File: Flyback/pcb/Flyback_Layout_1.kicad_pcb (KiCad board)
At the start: 2 copper layers, 44 parts

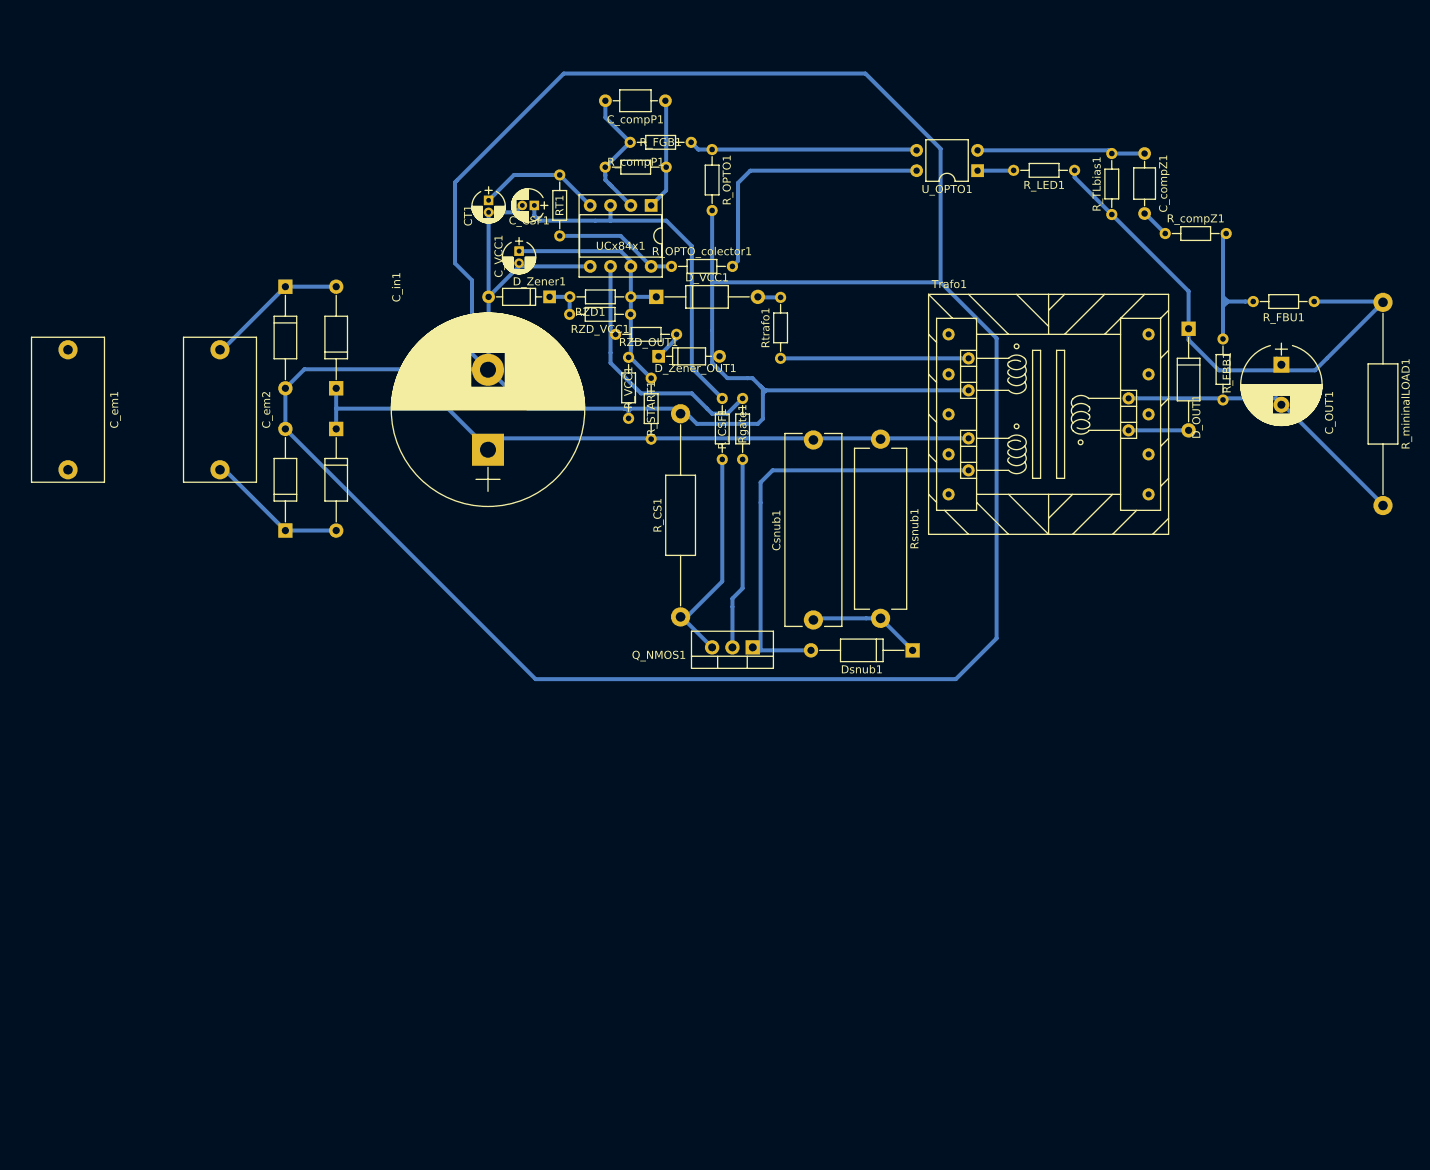
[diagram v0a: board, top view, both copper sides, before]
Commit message: add photo
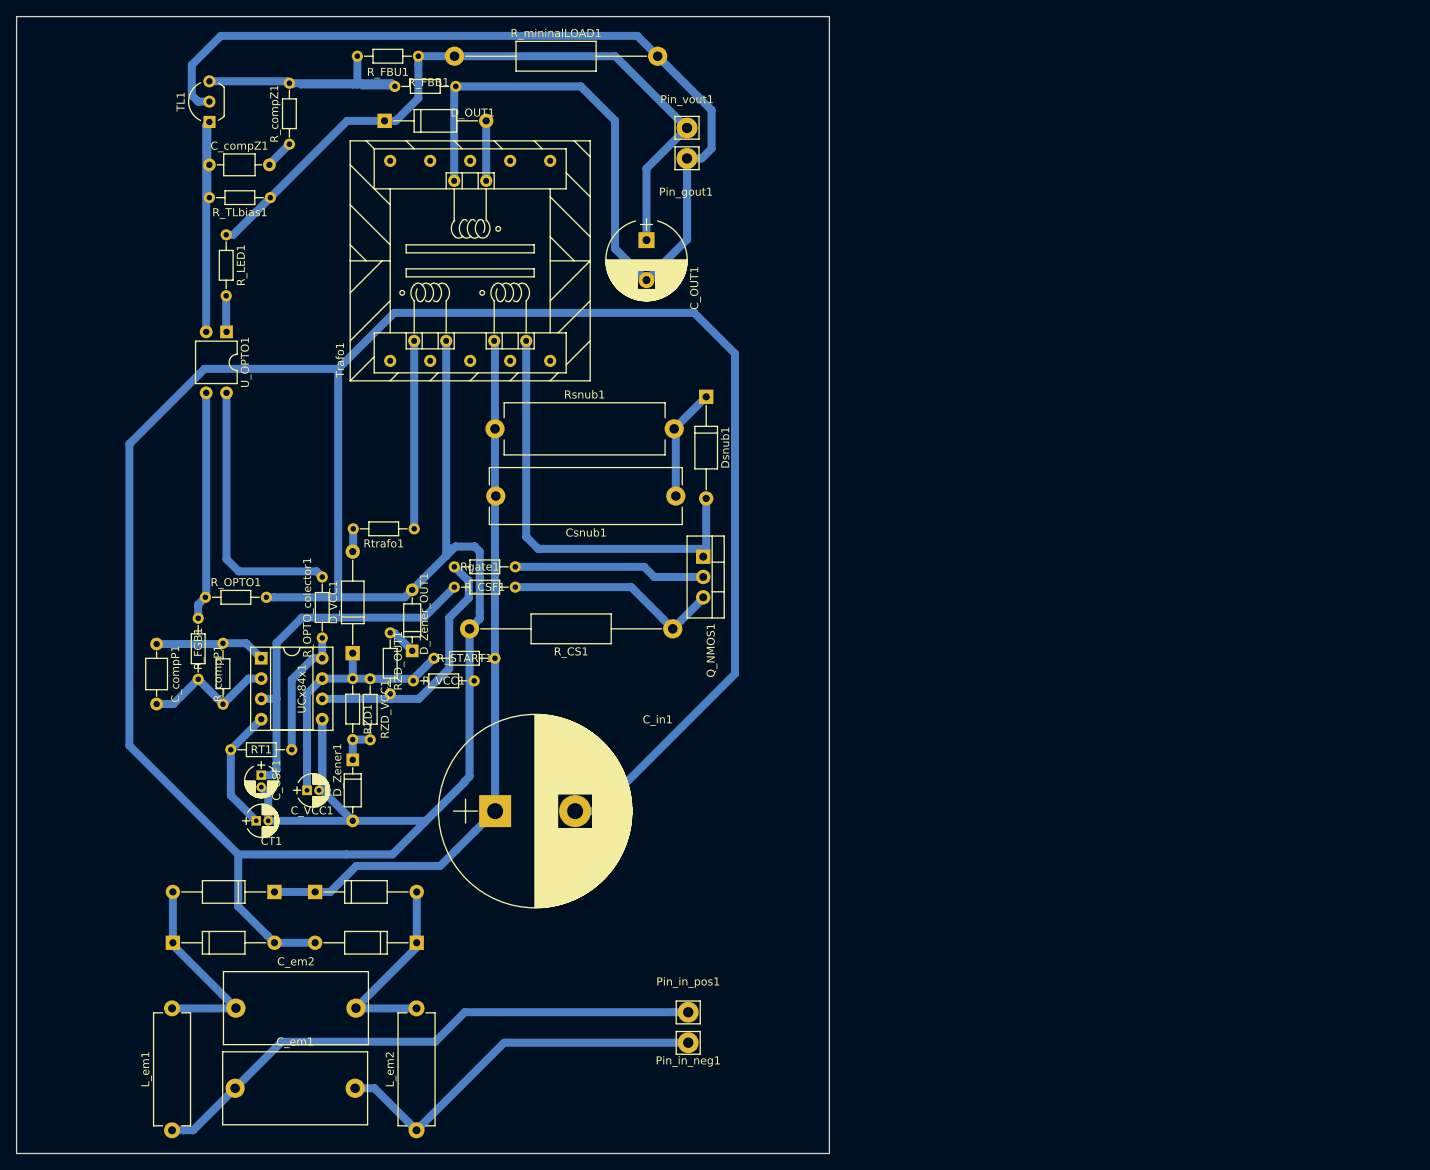
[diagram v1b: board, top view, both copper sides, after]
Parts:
- added L_em1: L, Inductors_THT:L_Axial_L14.0mm_D4.5mm_P15.24mm_Horizontal_Fastron_LACC, F.Cu at (75.4, 196.3)
- added L_em2: L, Inductors_THT:L_Axial_L14.0mm_D4.5mm_P15.24mm_Horizontal_Fastron_LACC, F.Cu at (105.9, 196.3)
- added Pin_gout1: CONN_01X01, Connectors:Pin_d1.4mm_L8.5mm_W2.8mm_FlatFork, F.Cu at (139.7, 74.8)
- added Pin_in_neg1: CONN_01X01, Connectors:Pin_d1.4mm_L8.5mm_W2.8mm_FlatFork, F.Cu at (139.9, 185.3)
- added Pin_in_pos1: CONN_01X01, Connectors:Pin_d1.4mm_L8.5mm_W2.8mm_FlatFork, F.Cu at (139.9, 181.5)
- added Pin_vout1: CONN_01X01, Connectors:Pin_d1.4mm_L8.5mm_W2.8mm_FlatFork, F.Cu at (139.7, 71.0)
- added TL1: Ajus_Shunt, TO_SOT_Packages_THT:TO-92_Inline_Wide, F.Cu at (80.0, 70.2)
- moved R_mininalLOAD1 120.1 mm to (110.7, 62.0), turned to 0 degrees
- moved C_compZ1 116.9 mm to (80.0, 75.6), turned to 0 degrees
- moved R_FBU1 116.1 mm to (98.5, 62.0)
- moved R_compZ1 110.0 mm to (90.0, 73.0), turned to 90 degrees
- moved R_LED1 106.4 mm to (82.1, 84.3), turned to 270 degrees
- moved R_TLbias1 105.2 mm to (87.7, 79.7), turned to 180 degrees
- moved D_OUT1 103.8 mm to (101.9, 70.1), turned to 0 degrees
- moved R_FBB1 103.6 mm to (110.8, 65.8), turned to 180 degrees
- moved U_OPTO1 96.0 mm to (82.2, 96.5), turned to 270 degrees
- moved C_em1 94.7 mm to (83.3, 191.0), turned to 0 degrees
- moved C_compP1 93.0 mm to (73.4, 135.5), turned to 270 degrees
- moved R_FGB1 86.1 mm to (78.6, 139.9), turned to 90 degrees
- moved R_OPTO1 84.5 mm to (79.5, 129.6), turned to 0 degrees
- moved Dret_1 83.2 mm to (75.5, 172.8), turned to 0 degrees
- moved CT1 82.8 mm to (85.9, 157.6), turned to 0 degrees
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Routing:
- net GOUT: track 37.3 -> 167.8 mm
- net Net-(C_em1-Pad1): track 0.00 -> 98.8 mm
- net VRET: track 88.7 -> 152.7 mm
- net Net-(C_em1-Pad2): track 0.00 -> 48.4 mm
- net GND: track 458.9 -> 499.2 mm
- net Net-(C_compZ1-Pad1): track 21.0 -> 52.8 mm
- net Net-(R_FBB1-Pad2): track 19.3 -> 46.7 mm
- net Net-(R_FGB1-Pad2): track 28.0 -> 53.6 mm
- net VOUT: track 65.2 -> 89.8 mm
- net ISENSE: track 45.1 -> 60.9 mm
- net VCC: track 33.3 -> 48.3 mm
- net Net-(C_em2-Pad1): track 17.8 -> 25.8 mm
- net Net-(C_em2-Pad2): track 17.7 -> 25.3 mm
- net DRENO: track 54.2 -> 60.5 mm
- net Net-(Q_NMOS1-Pad3): track 26.7 -> 32.5 mm
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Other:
- board outline added: 101.6 x 142.1 mm
- net class Default: trace_width 0.5 -> 1
